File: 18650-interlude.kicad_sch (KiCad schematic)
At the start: 4 parts, among them J1 PAD, J2 PAD, J3 CON

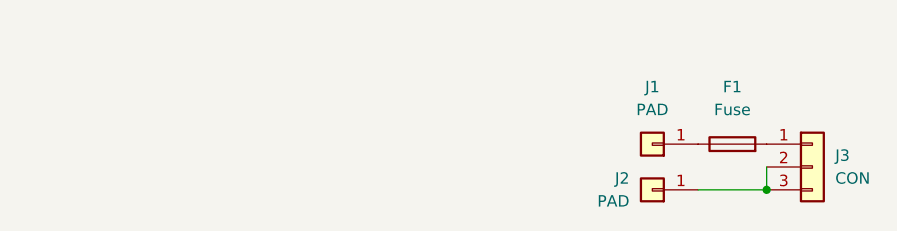
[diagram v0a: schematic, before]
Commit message: added schematic
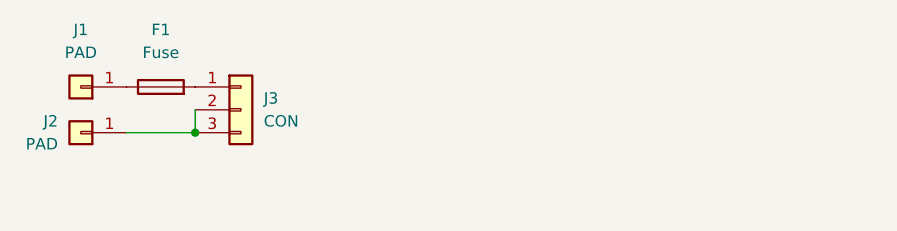
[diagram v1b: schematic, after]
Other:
- company: (none) -> Jana Marie Hemsing
- title: (none) -> 18650-interlude
- moved on the sheet: F1, J1, J2, J3
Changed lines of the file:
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@@
 (kicad_sch (version 20211123) (generator eeschema)
-  (paper "A4")
-  (junction (at 165.1 73.66) (diameter 0) (color 0 0 0 0)
+  (paper "A5")
+  (title_block
+    (title "18650-interlude")
+    (date "2022-11-27")
+    (rev "v1.1")
+    (company "Jana Marie Hemsing")
   )
-  (wire (pts (xy 165.1 71.12) (xy 165.1 73.66))
+  (junction (at 101.6 67.31) (diameter 0) (color 0 0 0 0)
+  )
+  (wire (pts (xy 101.6 64.77) (xy 101.6 67.31))
     (stroke (width 0) (type default) (color 0 0 0 0))
   )
-  (wire (pts (xy 165.1 73.66) (xy 157.48 73.66))
+  (wire (pts (xy 101.6 67.31) (xy 93.98 67.31))
     (stroke (width 0) (type default) (color 0 0 0 0))
   )
-  (symbol (lib_id "Connector_Generic:Conn_01x03") (at 170.18 71.12 0) (unit 1)
+  (symbol (lib_id "Connector_Generic:Conn_01x03") (at 106.68 64.77 0) (unit 1)
     (in_bom yes) (on_board yes) (fields_autoplaced)
-    (property "Reference" "J3" (id 0) (at 172.72 69.8499 0)
+    (property "Reference" "J3" (id 0) (at 109.22 63.4999 0)
       (effects (font (size 1.27 1.27)) (justify left))
     )
-    (property "Value" "CON" (id 1) (at 172.72 72.3899 0)
+    (property "Value" "CON" (id 1) (at 109.22 66.0399 0)
       (effects (font (size 1.27 1.27)) (justify left))
     )
-    (property "Footprint" "Connector_PinHeader_2.54mm:PinHeader_1x03_P2.54mm_Vertical" (id 2) (at 170.18 71.12 0)
+    (property "Footprint" "Connector_PinHeader_2.54mm:PinHeader_1x03_P2.54mm_Vertical" (id 2) (at 106.68 64.77 0)
       (effects (font (size 1.27 1.27)) hide)
     )
-    (property "Datasheet" "~" (id 3) (at 170.18 71.12 0)
+    (property "Datasheet" "~" (id 3) (at 106.68 64.77 0)
       (effects (font (size 1.27 1.27)) hide)
     )
@@
     (pin "3")
   )
-  (symbol (lib_id "Connector_Generic:Conn_01x01") (at 152.4 68.58 180) (unit 1)
+  (symbol (lib_id "Connector_Generic:Conn_01x01") (at 88.9 62.23 180) (unit 1)
     (in_bom yes) (on_board yes)
-    (property "Reference" "J1" (id 0) (at 152.4 62.23 0))
-    (property "Value" "PAD" (id 1) (at 152.4 64.77 0))
-    (property "Footprint" "otter:18650-pad" (id 2) (at 152.4 68.58 0)
+    (property "Reference" "J1" (id 0) (at 88.9 55.88 0))
+    (property "Value" "PAD" (id 1) (at 88.9 58.42 0))
+    (property "Footprint" "otter:18650-pad" (id 2) (at 88.9 62.23 0)
       (effects (font (size 1.27 1.27)) hide)
     )
-    (property "Datasheet" "~" (id 3) (at 152.4 68.58 0)
+    (property "Datasheet" "~" (id 3) (at 88.9 62.23 0)
       (effects (font (size 1.27 1.27)) hide)
     )
     (pin "1")
   )
-  (symbol (lib_id "Device:Fuse") (at 161.29 68.58 90) (unit 1)
+  (symbol (lib_id "Device:Fuse") (at 97.79 62.23 90) (unit 1)
     (in_bom yes) (on_board yes) (fields_autoplaced)
-    (property "Reference" "F1" (id 0) (at 161.29 62.23 90))
-    (property "Value" "Fuse" (id 1) (at 161.29 64.77 90))
-    (property "Footprint" "otter:R_0805" (id 2) (at 161.29 70.358 90)
+    (property "Reference" "F1" (id 0) (at 97.79 55.88 90))
+    (property "Value" "Fuse" (id 1) (at 97.79 58.42 90))
+    (property "Footprint" "otter:R_0805" (id 2) (at 97.79 64.008 90)
       (effects (font (size 1.27 1.27)) hide)
     )
-    (property "Datasheet" "~" (id 3) (at 161.29 68.58 0)
+    (property "Datasheet" "~" (id 3) (at 97.79 62.23 0)
       (effects (font (size 1.27 1.27)) hide)
     )
@@
     (pin "2")
   )
-  (symbol (lib_id "Connector_Generic:Conn_01x01") (at 152.4 73.66 180) (unit 1)
+  (symbol (lib_id "Connector_Generic:Conn_01x01") (at 88.9 67.31 180) (unit 1)
     (in_bom yes) (on_board yes) (fields_autoplaced)
-    (property "Reference" "J2" (id 0) (at 149.86 72.3899 0)
+    (property "Reference" "J2" (id 0) (at 86.36 66.0399 0)
       (effects (font (size 1.27 1.27)) (justify left))
     )
-    (property "Value" "PAD" (id 1) (at 149.86 74.9299 0)
+    (property "Value" "PAD" (id 1) (at 86.36 68.5799 0)
       (effects (font (size 1.27 1.27)) (justify left))
     )
-    (property "Footprint" "otter:18650-pad" (id 2) (at 152.4 73.66 0)
+    (property "Footprint" "otter:18650-pad" (id 2) (at 88.9 67.31 0)
       (effects (font (size 1.27 1.27)) hide)
     )
-    (property "Datasheet" "~" (id 3) (at 152.4 73.66 0)
+    (property "Datasheet" "~" (id 3) (at 88.9 67.31 0)
       (effects (font (size 1.27 1.27)) hide)
     )
